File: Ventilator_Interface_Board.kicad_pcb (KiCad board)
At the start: 2 copper layers, 60 x 88.5 mm, 53 parts, among them J1 ROTARY CONTROLS, J3 ALARM, J4 LCD DISPLAY, J5 OPTICAL SWITCH, J6 HOME LIMIT SWITCH, P1 Power, P2 Analog, P3 Digital, P4 Digital, P5 CONN_01X01, P6 CONN_01X01, P7 CONN_01X01, P8 CONN_01X01, SW1 SW_Push, U1 HSCMRRN100MDAA5, U2 HSCDRRN100MDAA5

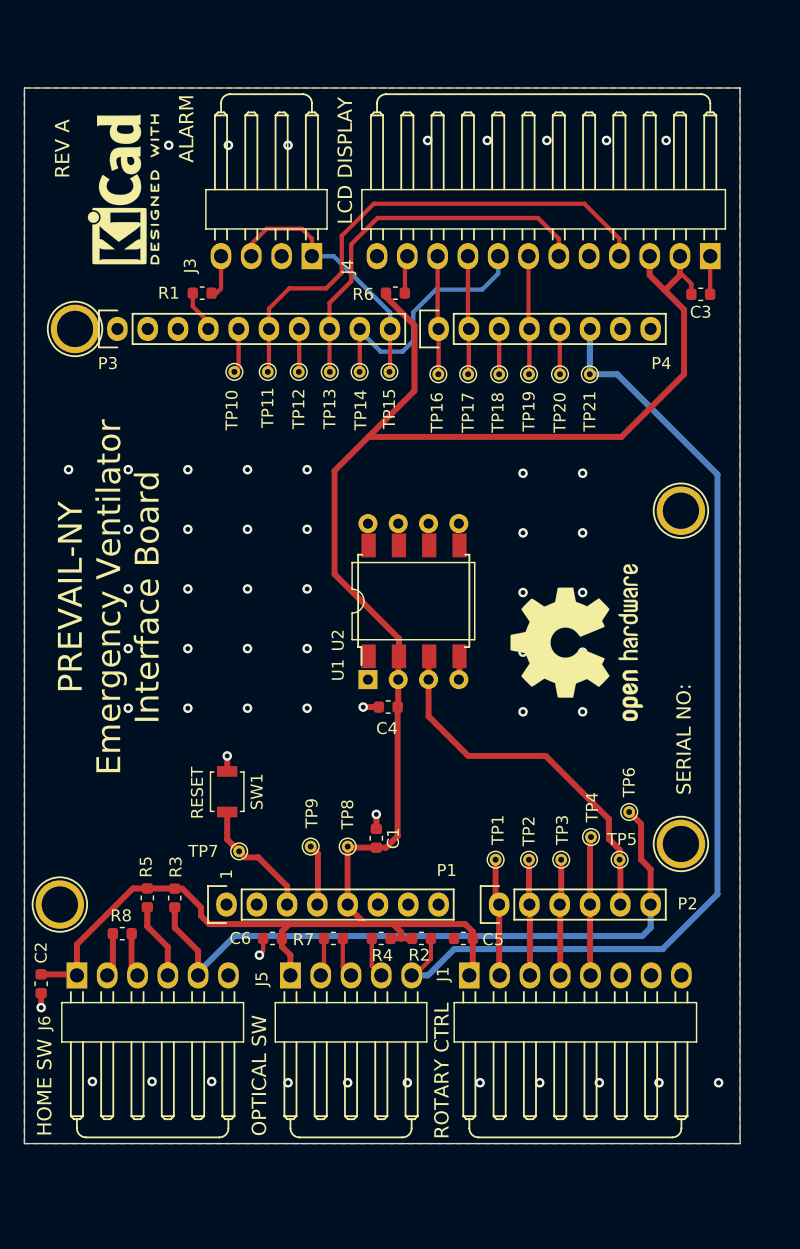
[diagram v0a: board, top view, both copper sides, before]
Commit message: Rev A - pre-release
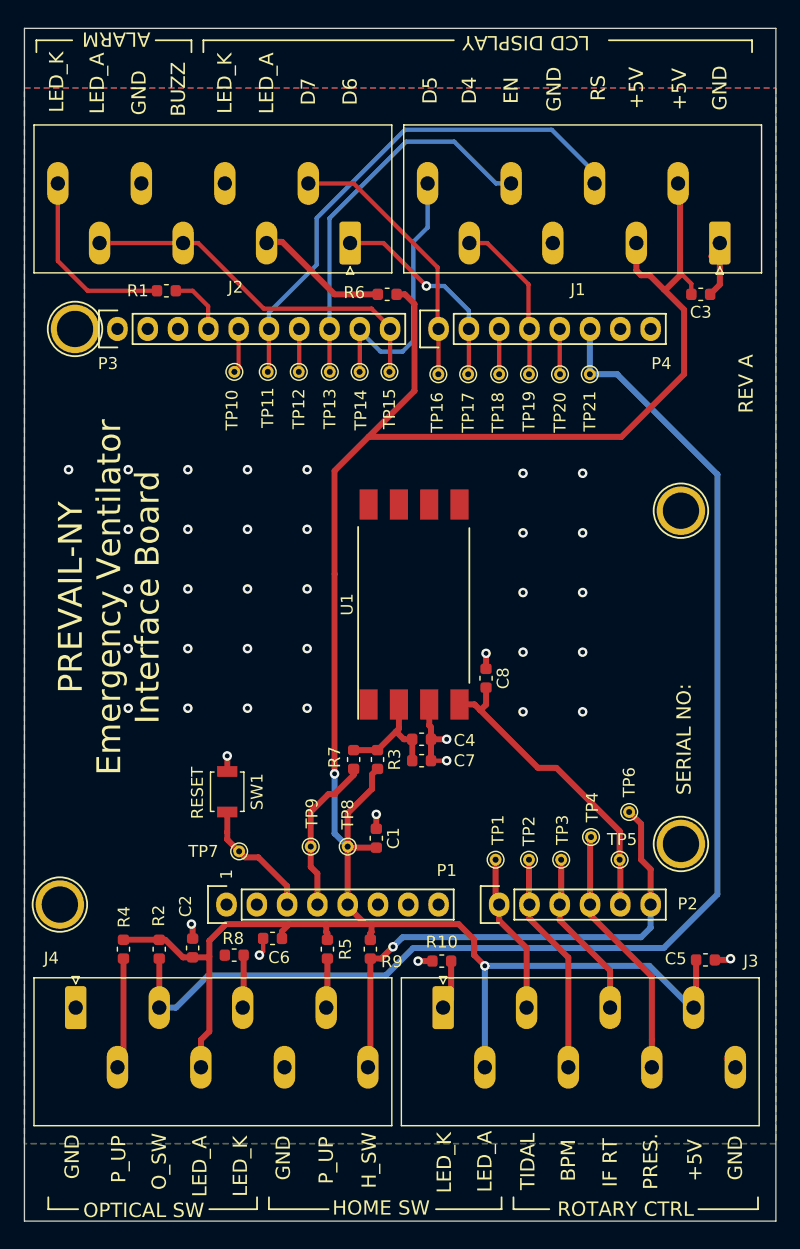
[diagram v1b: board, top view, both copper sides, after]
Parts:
- removed J5: OPTICAL SWITCH, Ventilator:Molex_KK-254_1x05_P2.54mm_Horizontal
- removed J6: HOME LIMIT SWITCH, Ventilator:Molex_KK-254_1x06_P2.54mm_Horizontal
- removed REF**: KiCad-Logo2_6mm_SilkScreen, Symbol:KiCad-Logo2_6mm_SilkScreen
- removed REF**: OSHW-Logo2_14.6x12mm_SilkScreen, Symbol:OSHW-Logo2_14.6x12mm_SilkScreen
- removed U2: HSCDRRN100MDAA5, Ventilator:DIP-8_W13.08mm
- added C7: 1uF, Capacitor_SMD:C_0603_1608Metric, F.Cu at (155.3, 111.8)
- added C8: 470pF, Capacitor_SMD:C_0603_1608Metric, F.Cu at (160.7, 104.9)
- added J2: Conn_01x08, Ventilator:PhoenixContact_PTSA_1,5_8-3_5-Z_1x08_P3.50mm_Vertical, F.Cu at (149.3, 68.4)
- added R10: 330R, Resistor_SMD:R_0603_1608Metric, F.Cu at (157.0, 128.6)
- added R9: 10K, Resistor_SMD:R_0603_1608Metric, F.Cu at (151.0, 127.6)
- J1: value ROTARY CONTROLS -> Conn_01x08; footprint Ventilator:Molex_KK-254_1x08_P2.54mm_Horizontal -> Ventilator:PhoenixContact_PTSA_1,5_8-3_5-Z_1x08_P3.50mm_Vertical
- J3: value ALARM -> Conn_01x08; footprint Ventilator:Molex_KK-254_1x04_P2.54mm_Horizontal -> Ventilator:PhoenixContact_PTSA_1,5_8-3_5-Z_1x08_P3.50mm_Vertical
- J4: value LCD DISPLAY -> Conn_01x08; footprint Ventilator:Molex_KK-254_1x12_P2.54mm_Horizontal -> Ventilator:PhoenixContact_PTSA_1,5_8-3_5-Z_1x08_P3.50mm_Vertical
- R3: value 10K -> DNF
- R7: value 330R -> 0R
- U1: value HSCMRRN100MDAA5 -> MP3V5004GP; footprint Ventilator:SMT-8W_7.5x8.8mm_P2.54mm -> Ventilator:SOP_16.8x7.62mm_P2.54mm
- moved J4 82.5 mm to (126.3, 132.5), turned to 0 degrees
- moved J1 64.9 mm to (180.3, 68.4), turned to 180 degrees
- moved J3 64.0 mm to (157.1, 132.5), turned to 0 degrees
- moved R2 22.0 mm to (133.3, 127.6), turned to 90 degrees
- moved R4 21.6 mm to (130.3, 127.6), turned to 90 degrees
- moved R3 20.6 mm to (151.6, 111.7)
- moved C5 20.4 mm to (179.1, 128.5), turned to 180 degrees
- moved R5 15.7 mm to (147.4, 127.6), turned to 90 degrees
- moved R7 15.1 mm to (149.6, 111.7), turned to 270 degrees
- moved C2 13.0 mm to (136.1, 127.5), turned to 270 degrees
- moved R8 9.56 mm to (139.6, 128.1), turned to 180 degrees
- moved C4 3.89 mm to (155.3, 110.0), turned to 180 degrees
- moved R1 3.01 mm to (133.9, 72.4), turned to 0 degrees
- moved R6 0.69 mm to (152.4, 72.7), turned to 0 degrees
- moved U1 0.30 mm to (155.3, 98.7)
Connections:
- C4 pad 2: +5V -> Net-(C4-Pad2)
- J1 pad 1: +5V -> GND
- J1 pad 2: /TIDAL_VOLUME -> +5V
- J1 pad 3: /BPM -> +5V
- J1 pad 4: /IF_RATE -> /LCD_RS
- J1 pad 5: /MAX_PRESSURE -> GND
- J1 pad 6: GND -> /LCD_EN
- J1 pad 7: (no net) -> /LCD_D4
- J1 pad 8: (no net) -> /LCD_D5
- J3 pad 1: /BUZZER_LED -> Net-(J3-Pad1)
- J3 pad 2: GND -> +5V
- J3 pad 3: /BUZZER_LED -> /TIDAL_VOLUME
- J3 pad 4: Net-(J3-Pad4) -> /BPM
- J4 pad 2: +5V -> Net-(J4-Pad2)
- J4 pad 3: +5V -> /OPTICAL_SW
- J4 pad 4: /LCD_RS -> +5V
- J4 pad 5: GND -> Net-(J4-Pad5)
- J4 pad 6: /LCD_EN -> GND
- J4 pad 7: /LCD_D4 -> Net-(J4-Pad7)
- J4 pad 8: /LCD_D5 -> /HOME_LIMIT_SW
- R1 pad 1: Net-(J3-Pad4) -> Net-(J2-Pad8)
- R2 pad 1: +5V -> /OPTICAL_SW
- R2 pad 2: /OPTICAL_SW -> +5V
- R3 pad 1: +5V -> Net-(C4-Pad2)
- R3 pad 2: /HOME_LIMIT_SW -> +5V
- R4 pad 1: +5V -> Net-(J4-Pad2)
- R4 pad 2: Net-(J5-Pad4) -> +5V
- R5 pad 1: +5V -> Net-(J4-Pad7)
- R5 pad 2: Net-(J6-Pad4) -> +5V
- R6 pad 1: Net-(J4-Pad11) -> Net-(J2-Pad3)
- R7 pad 1: Net-(J5-Pad2) -> Net-(C4-Pad2)
- R7 pad 2: GND -> +3V3
- R8 pad 1: Net-(J6-Pad2) -> Net-(J4-Pad5)
- U1 pad 2: +5V -> Net-(C4-Pad2)
- U1 pad 3: /PRESSURE_SENSOR -> GND
- U1 pad 4: GND -> /PRESSURE_SENSOR
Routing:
- net +5V: track 164.7 -> 202.9 mm, vias 0 -> 2
- net /OPTICAL_SW: track 85.6 -> 108.0 mm
- net Net-(J2-Pad8): track 0.00 -> 15.8 mm
- net /LCD_D7: track 9.94 -> 22.8 mm
- net /HOME_LIMIT_SW: track 56.7 -> 44.2 mm, vias 0 -> 1
- net Net-(J2-Pad3): track 0.00 -> 11.2 mm
- net Net-(C4-Pad2): track 0.00 -> 10.00 mm
- net /MAX_PRESSURE: track 11.6 -> 21.5 mm
- net Net-(J4-Pad2): track 0.00 -> 9.32 mm
- net /BUZZER_LED: track 22.0 -> 31.1 mm
- net /BPM: track 9.73 -> 18.8 mm
- net +3V3: track 5.13 -> 13.4 mm
- net /LCD_D6: track 9.96 -> 17.8 mm, vias 0 -> 1
- net Net-(J6-Pad4): track 6.42 -> 0.00 mm
- net /PRESSURE_SENSOR: track 31.3 -> 26.1 mm
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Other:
- board size 60 x 88.5 mm -> 63 x 100 mm
- board text added: "+5V"
- board text added: "BPM"
- board text added: "BUZZ"
- board text added: "D4"
- board text added: "D5"
- board text added: "D6"
- board text added: "D7"
- board text added: "EN"
- board text added: "GND"
- board text added: "H_SW"
- board text added: "IF RT"
- board text added: "LED_A"
- board text added: "LED_K"
- board text added: "O_SW"
- board text added: "PRES."
- board text added: "P_UP"
- board text added: "RS"
- board text added: "TIDAL"
